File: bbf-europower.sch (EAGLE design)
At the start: 13 parts, among them J1 CON_HEADER_2X05-PTH, J2 CON_HEADER_2X05-PTH

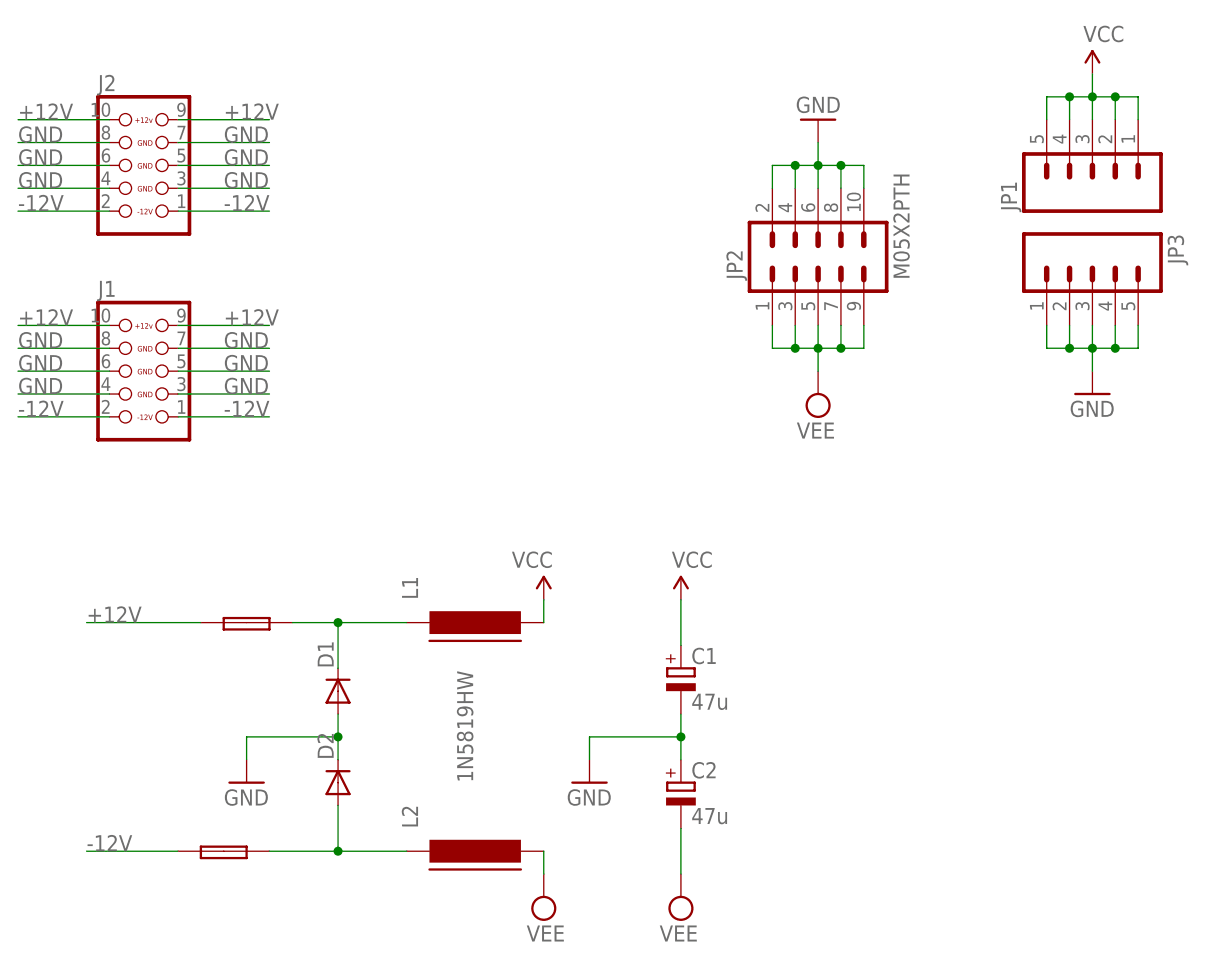
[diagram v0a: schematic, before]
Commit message: almost there
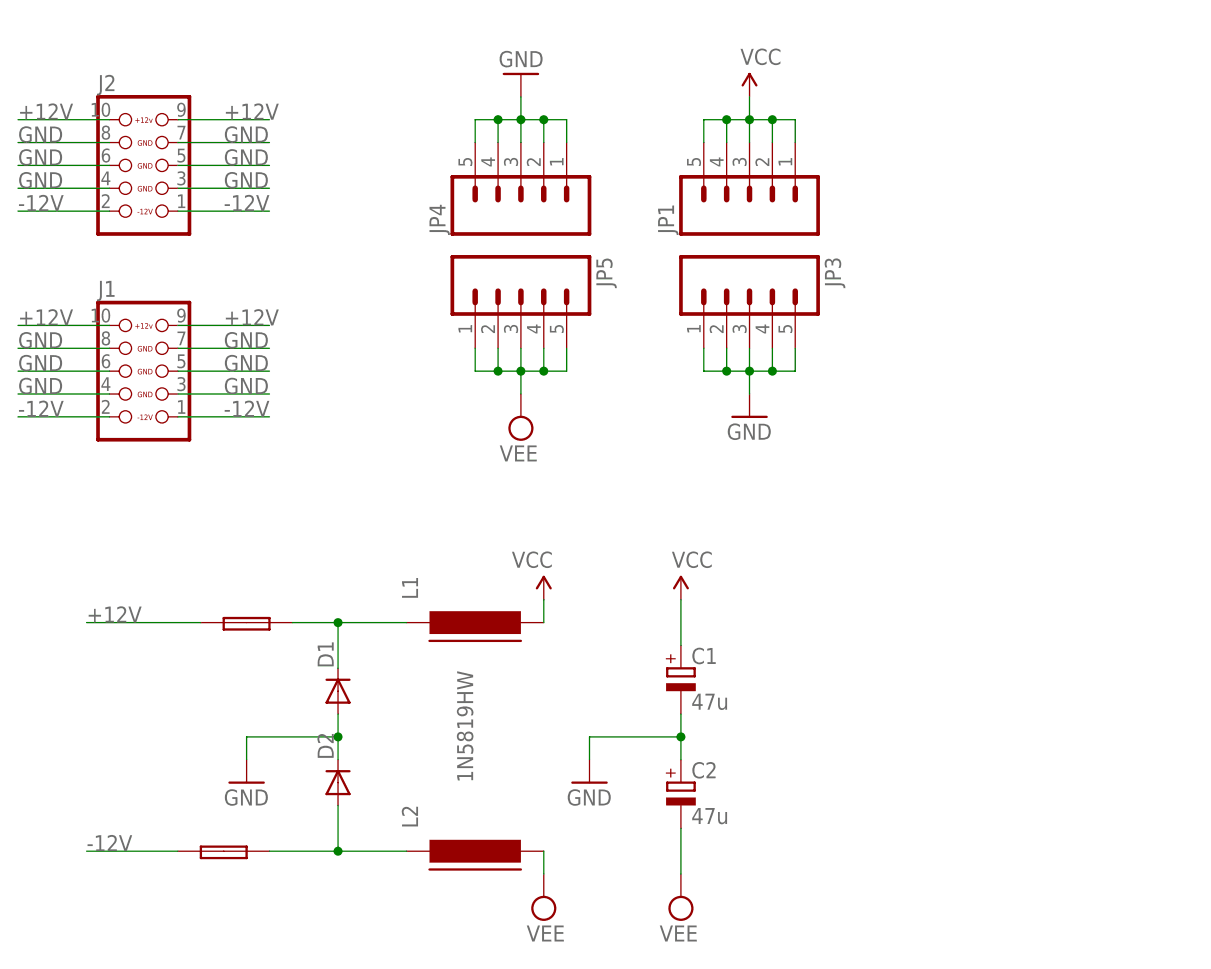
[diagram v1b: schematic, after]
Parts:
- removed JP2: M05X2PTH, SparkFun:M05X2PTH
- added JP4, JP5: (no value), SparkFun:M05PTH
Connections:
- net GND: now also JP4.1, JP4.2, JP4.3, JP4.4, JP4.5; no longer JP2.10, JP2.2, JP2.4, JP2.6, JP2.8
- net VEE: now also JP5.1, JP5.2, JP5.3, JP5.4, JP5.5; no longer JP2.1, JP2.3, JP2.5, JP2.7, JP2.9
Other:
- moved on the sheet: JP1, JP3
